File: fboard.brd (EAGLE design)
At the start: 48.2 x 60.6 mm, 41 parts, among them U1 ATMEGA328PB-AU, U2 MPU-6050

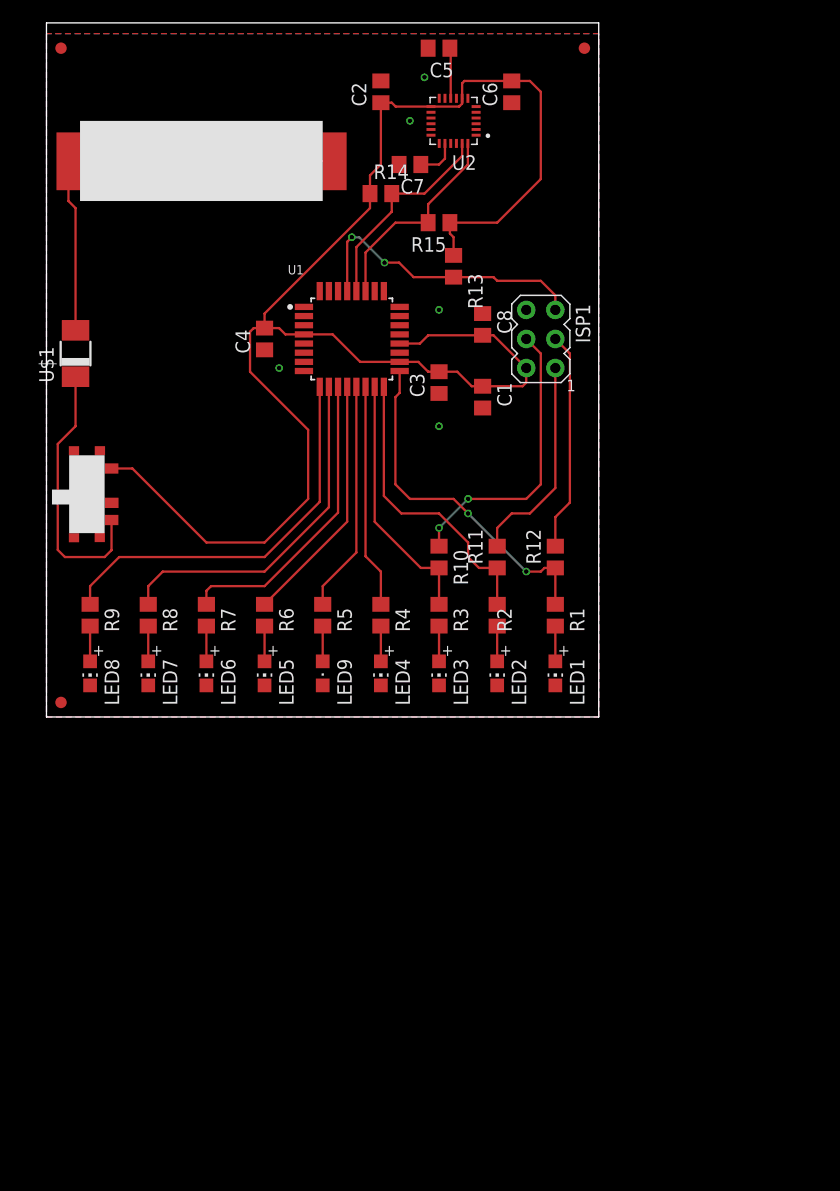
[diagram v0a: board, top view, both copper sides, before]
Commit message: fixed schematic
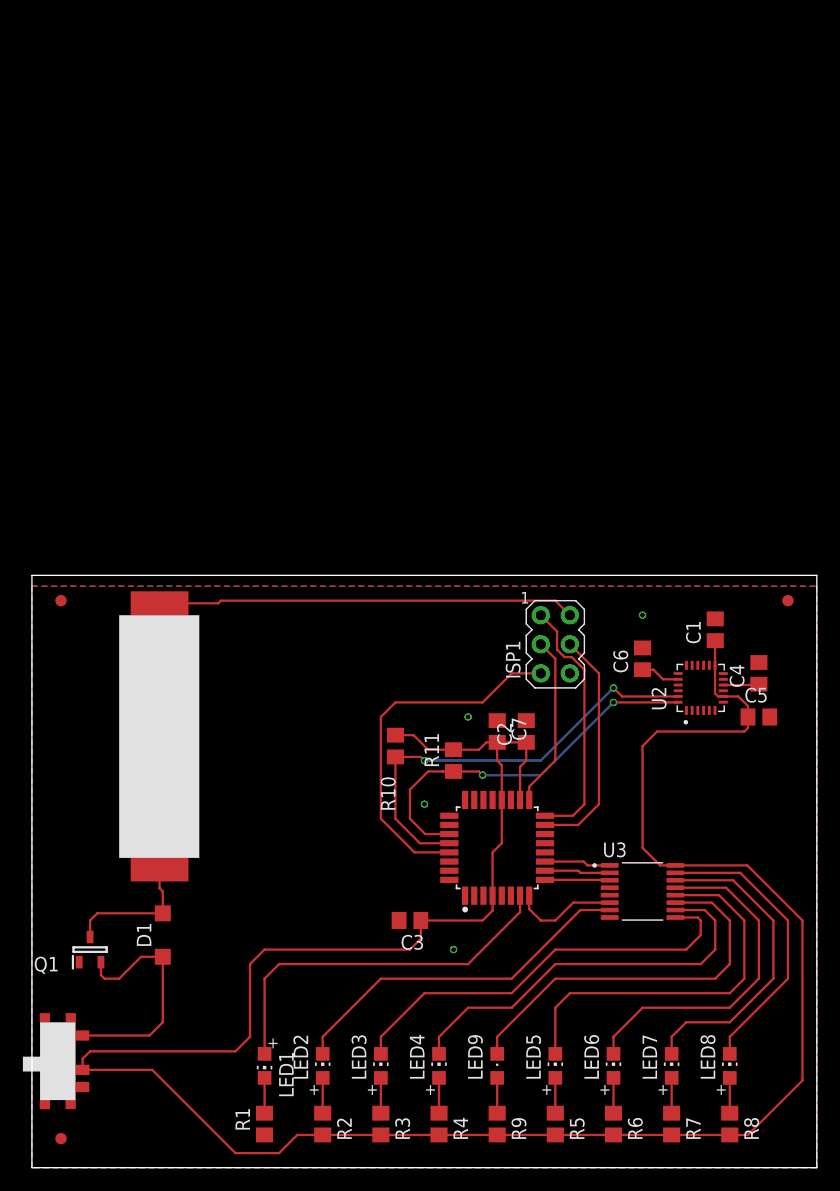
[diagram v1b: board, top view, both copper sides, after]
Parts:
- removed C8: 0.1uF, rcl:C0805
- removed R12: 330R, rcl:R0805
- removed R13: 2.7kR, rcl:R0805
- removed R14, R15: 4.7kR, rcl:R0805
- removed U$1: SS14, SS14:DO-214AC
- removed U$2: SK-3296S-01-L1, CustomParts:SK-3296S-01-L1
- removed U$3: RK-2032, CustomParts:RK-2032
- added BAT1: RK-2032, CustomParts:RK-2032
- added D1: MBR0520LT, diode:SOD123
- added Q1: SL2305, SL2305:SOT95P240X115-3N
- added S1: SK-3296S-01-L1, CustomParts:SK-3296S-01-L1
- added U3: SN74HC138PW, SN74HC138PW:SOP65P640X120-16N
- C5: value 0.1uF -> 10nF
- C6: value 10nF -> 2nF
- C7: value 2nF -> 0.1uF
- R10, R11: value 330R -> 4.7kR
- moved U$6 95.2 mm to (2.54, 2.54)
- moved R8 67.5 mm to (61.0, 3.81)
- moved LED8 65.6 mm to (61.0, 8.89), turned to 0 degrees
- moved C5 64.8 mm to (63.5, 39.4), turned to 0 degrees
- moved R7 60.2 mm to (55.9, 3.81)
- moved C2 57.3 mm to (43.2, 38.1)
- moved LED7 57.1 mm to (55.9, 8.89), turned to 0 degrees
- moved R9 56.9 mm to (40.6, 3.81)
- moved U2 54.0 mm to (58.4, 41.9), turned to 90 degrees
- moved R6 53.9 mm to (50.8, 3.81)
- moved C4 52.1 mm to (63.5, 43.2)
- moved U$5 51.4 mm to (66.0, 49.5)
- moved R1 51.2 mm to (20.3, 3.81), turned to 90 degrees
- moved C6 50.8 mm to (53.3, 44.5)
- moved C7 50.1 mm to (40.6, 38.1), turned to 270 degrees
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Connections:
- removed net B3: ISP1.4, R10.1
- removed net B4: ISP1.1, R11.2
- removed net B5: ISP1.3, R12.2
- removed net N$10: LED4.A, R4.2
- removed net N$11: LED9.A, R5.2
- removed net N$12: LED5.A, R6.2
- removed net N$13: LED6.A, R7.2
- removed net N$14: LED7.A, R8.2
- removed net N$15: LED8.A, R9.2
- removed net N$16: U$1.C, U$2.P3
- removed net N$2: LED1.A, R1.2
- removed net PB0: R6.1, U1.12
- removed net PB1: R5.1, U1.13
- removed net PB2: R4.1, U1.14
- removed net VOLTAGEPROTEC: U$1.A, U$3.P$1, U$3.P$2
- new net 3V_INPUT: BAT1.P$1, BAT1.P$2, D1.A, ISP1.2, Q1.3
- new net N$1: LED2.A, R2.1
- new net N$19: LED1.C, R1.2
- new net N$3: LED3.A, R3.1
- new net N$4: LED4.A, R4.1
- new net N$5: LED9.A, R9.1
- new net N$6: LED5.A, R5.1
- new net N$7: LED6.A, R6.1
- new net PB6: LED1.A, U1.7
- new net PB7: U1.8, U3.6
- new net VPROTEC: D1.C, Q1.2, S1.P1
- new net Y0: LED8.C, U3.15
- new net Y1: LED7.C, U3.14
- new net Y2: LED6.C, U3.13
- new net Y3: LED5.C, U3.12
- new net Y4: LED9.C, U3.11
- new net Y5: LED4.C, U3.10
- new net Y6: LED3.C, U3.9
- new net Y7: LED2.C, U3.7
- net CPOUT: now also C6.1; no longer C7.1
- net GND: now also BAT1.P$3, C3.2, C4.2, C6.2, C7.1, Q1.1, R1.1, S1.P3, U3.8; no longer C3.1, C4.1, C6.1, C7.2, C8.1, LED1.C, LED2.C, LED3.C, LED4.C, LED5.C, LED6.C, LED7.C, LED8.C, LED9.C, U$3.P$3
- net N$8: now also LED7.A, R7.1; no longer LED2.A, R2.2
- net N$9: now also LED8.A, R8.1; no longer LED3.A, R3.2
- net PB3: now also ISP1.4; no longer R10.2, R3.1
- net PB4: now also ISP1.1; no longer R11.1, R2.1
- net PB5: now also ISP1.3; no longer R1.1, R12.1
- net PC4: now also R11.1; no longer R15.2
- net PC5: now also R10.1; no longer R14.2
- net PC6: no longer R13.2
- net PD5: now also U3.3; no longer R9.1
- net PD6: now also U3.2; no longer R8.1
- net PD7: now also U3.1; no longer R7.1
- net REGOUT: now also C4.1; no longer C5.1
- net VCC: now also C3.1, C5.1, C7.2, R10.2, R11.2, R2.2, R3.2, R4.2, R5.2, R6.2, R7.2, R8.2, R9.2, S1.P2, U3.16; no longer C3.2, C4.2, C6.2, C8.2, ISP1.2, R13.1, R14.1, R15.1, U$2.P1
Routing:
- net 3V_INPUT: track 0.00 -> 73.6 mm
- net VCC: track 139.0 -> 207.5 mm
- net VOLTAGEPROTEC: track 40.1 -> 0.00 mm
- net Y6: track 0.00 -> 36.7 mm
- net Y5: track 0.00 -> 35.4 mm
- net Y4: track 0.00 -> 33.6 mm
- net Y3: track 0.00 -> 33.6 mm
- net PB6: track 0.00 -> 32.7 mm
- net Y7: track 0.00 -> 31.1 mm
- net Y2: track 0.00 -> 29.9 mm
- net PD5: track 34.7 -> 5.66 mm
- net Y1: track 0.00 -> 27.6 mm
- net Y0: track 0.00 -> 25.3 mm
- net B3: track 25.3 -> 0.00 mm, vias 2 -> 0
- net PD6: track 30.7 -> 5.73 mm
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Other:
- board size 48.2 x 60.6 mm -> 68.6 x 51.7 mm
